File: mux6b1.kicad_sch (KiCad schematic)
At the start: 7 parts, among them U1 4081, U10 4071, U18 4069, U27 4069, U46 4071, U48 4081, U6 4081

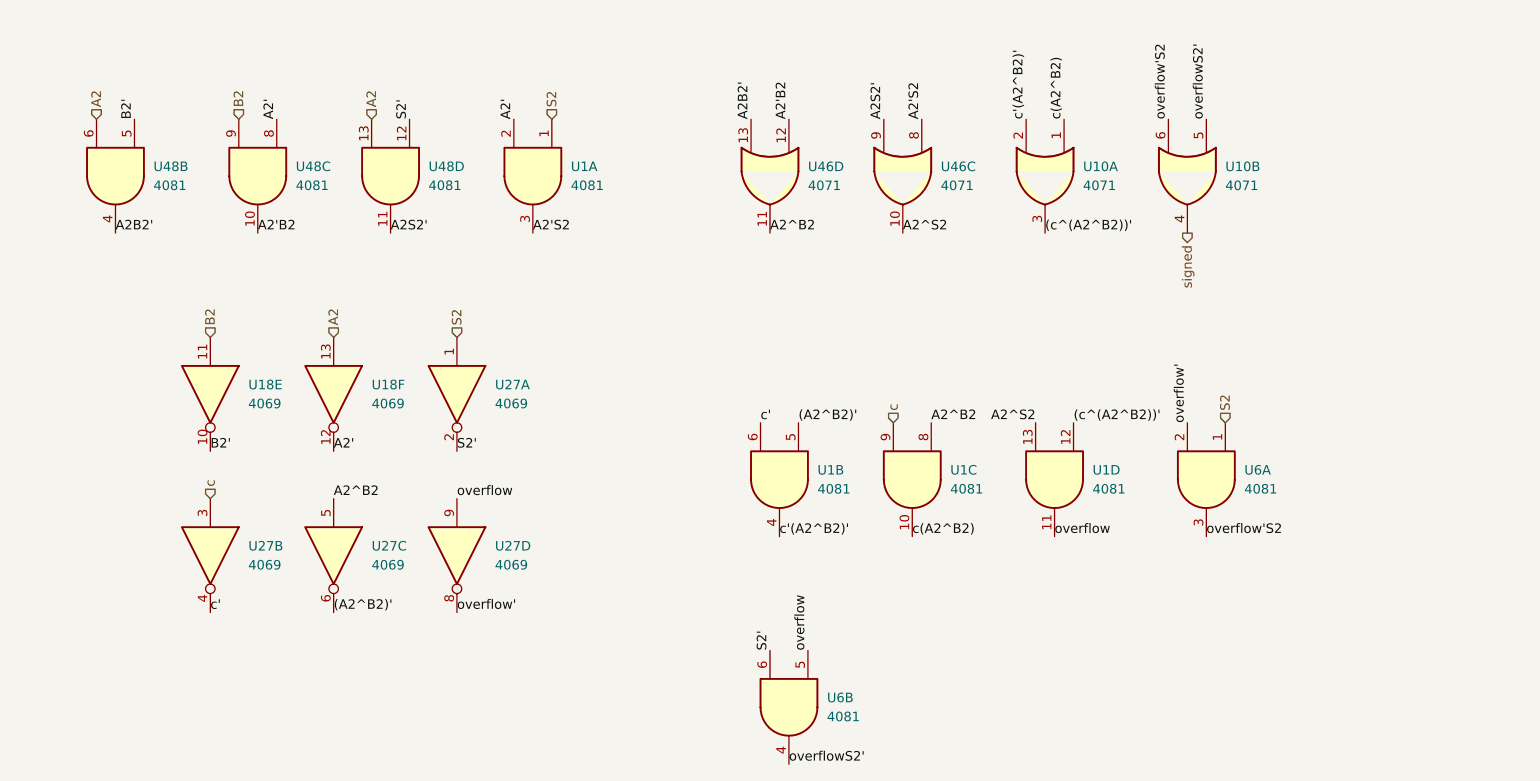
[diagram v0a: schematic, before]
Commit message: Add files via upload
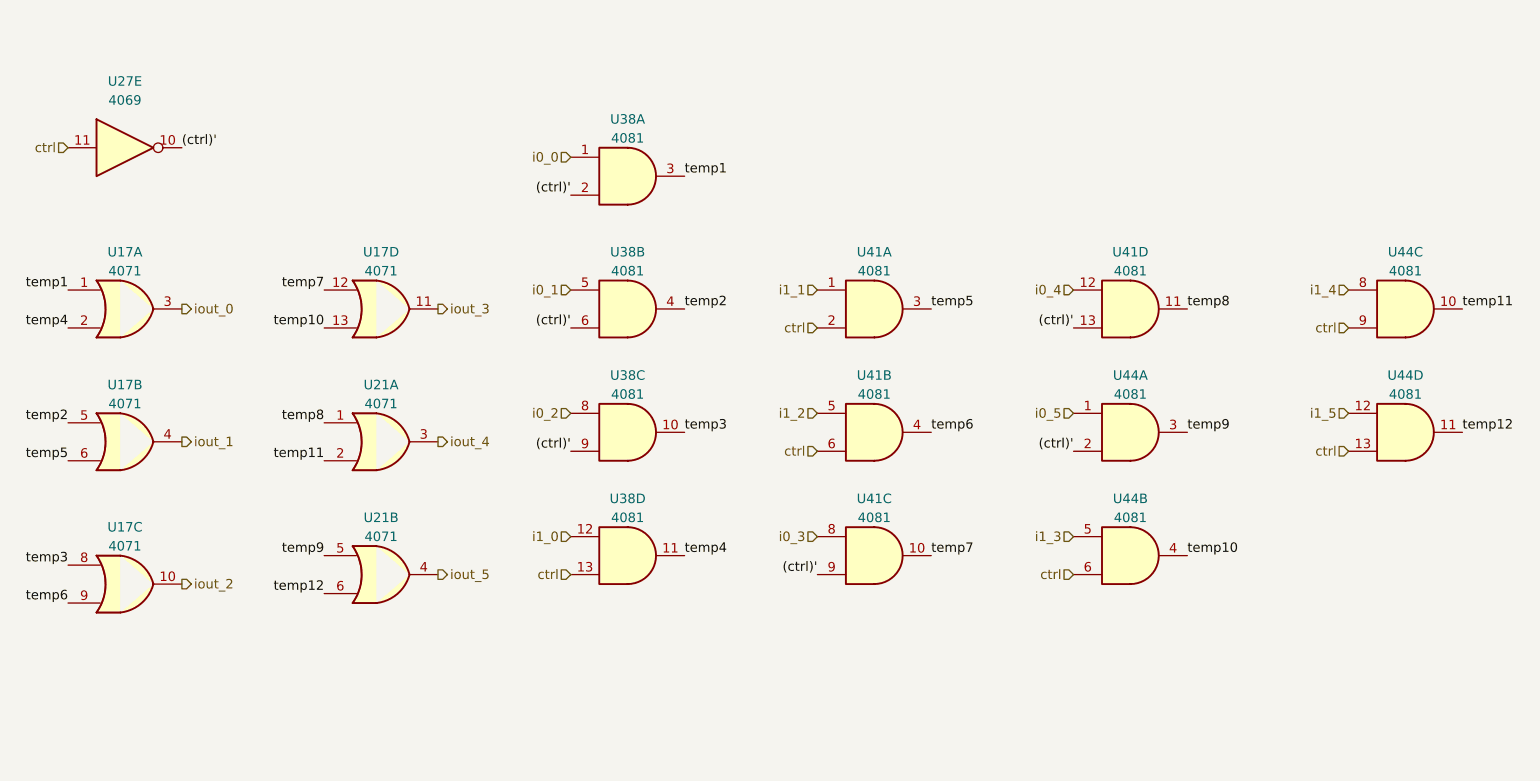
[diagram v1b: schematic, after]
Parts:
- removed U1, U48, U6: 4081, Package_DIP:CERDIP-14_W7.62mm_SideBrazed_LongPads_Socket, symbol 4xxx:4081
- removed U10, U46: 4071, Package_DIP:CERDIP-14_W7.62mm_SideBrazed_LongPads_Socket, symbol 4xxx:4071
- removed U18, U27: 4069, Package_DIP:CERDIP-14_W7.62mm_SideBrazed_LongPads_Socket, symbol 4xxx:4069
- added U17, U21: 4071, Package_DIP:CERDIP-14_W7.62mm_SideBrazed_LongPads_Socket, symbol 4xxx:4071
- added U27: 4069, Package_DIP:CERDIP-14_W7.62mm_SideBrazed_LongPads_Socket, symbol 4xxx:4069
- added U38, U41, U44: 4081, Package_DIP:CERDIP-14_W7.62mm_SideBrazed_LongPads_Socket, symbol 4xxx:4081
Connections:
- new net (ctrl)': U27.10, U38.2, U38.6, U38.9, U41.13, U41.9, U44.2
- new net ctrl: U27.11, U38.13, U41.2, U41.6, U44.13, U44.6, U44.9
- new net i0_0: U38.1
- new net i0_1: U38.5
- new net i0_2: U38.8
- new net i0_3: U41.8
- new net i0_4: U41.12
- new net i0_5: U44.1
- new net i1_0: U38.12
- new net i1_1: U41.1
- new net i1_2: U41.5
- new net i1_3: U44.5
- new net i1_4: U44.8
- new net i1_5: U44.12
- new net iout_0: U17.3
- new net iout_1: U17.4
- new net iout_2: U17.10
- new net iout_3: U17.11
- new net iout_4: U21.3
- new net iout_5: U21.4
- new net temp1: U17.1, U38.3
- new net temp10: U17.13, U44.4
- new net temp11: U21.2, U44.10
- new net temp12: U21.6, U44.11
- new net temp2: U17.5, U38.4
- new net temp3: U17.8, U38.10
- new net temp4: U17.2, U38.11
- new net temp5: U17.6, U41.3
- new net temp6: U17.9, U41.4
- new net temp7: U17.12, U41.10
- new net temp8: U21.1, U41.11
- new net temp9: U21.5, U44.3
